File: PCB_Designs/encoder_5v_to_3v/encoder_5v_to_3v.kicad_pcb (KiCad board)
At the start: 2 copper layers, 52.1 x 57.2 mm, 17 parts, among them J1 Screw_Terminal_01x02, J2 Screw_Terminal_01x02, J3 Screw_Terminal_01x02, J4 Screw_Terminal_01x02, J5 Screw_Terminal_01x02, J6 Screw_Terminal_01x02, J7 Screw_Terminal_01x02, J8 Screw_Terminal_01x02

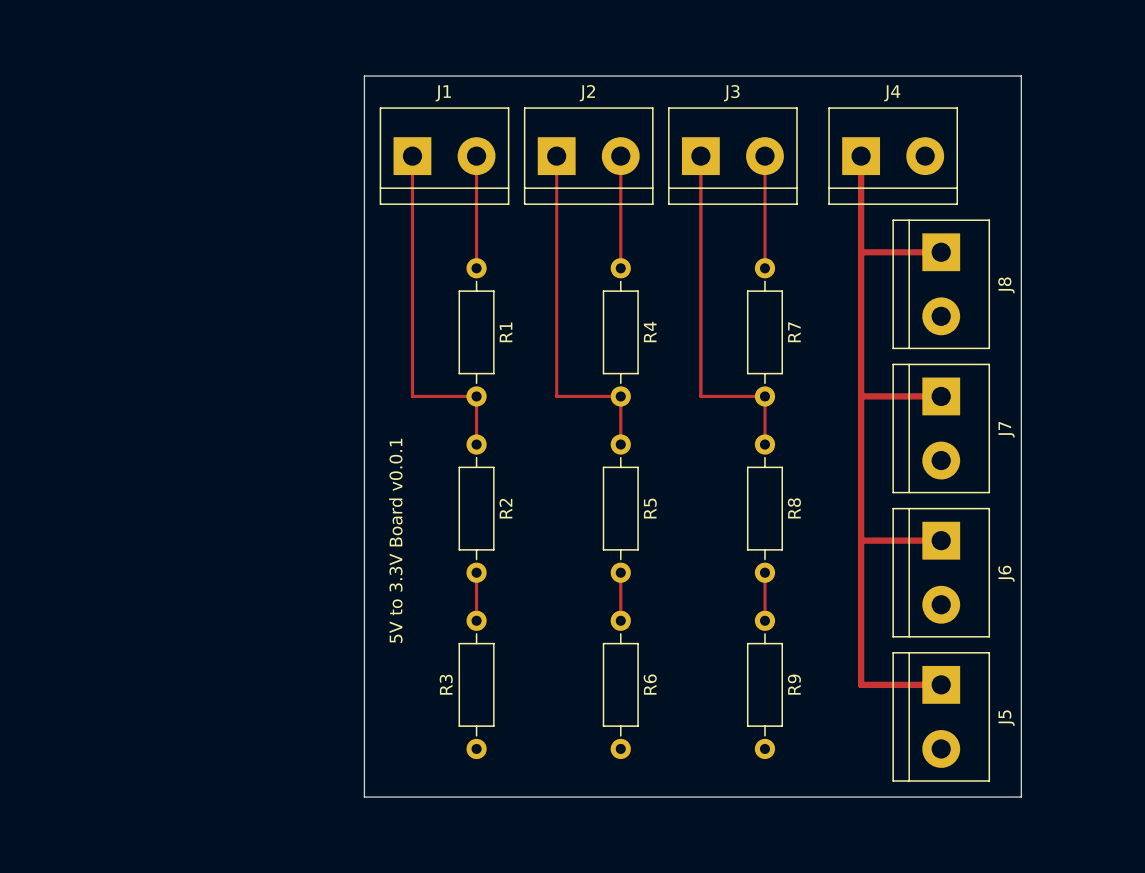
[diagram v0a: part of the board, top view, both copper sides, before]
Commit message: update PCB
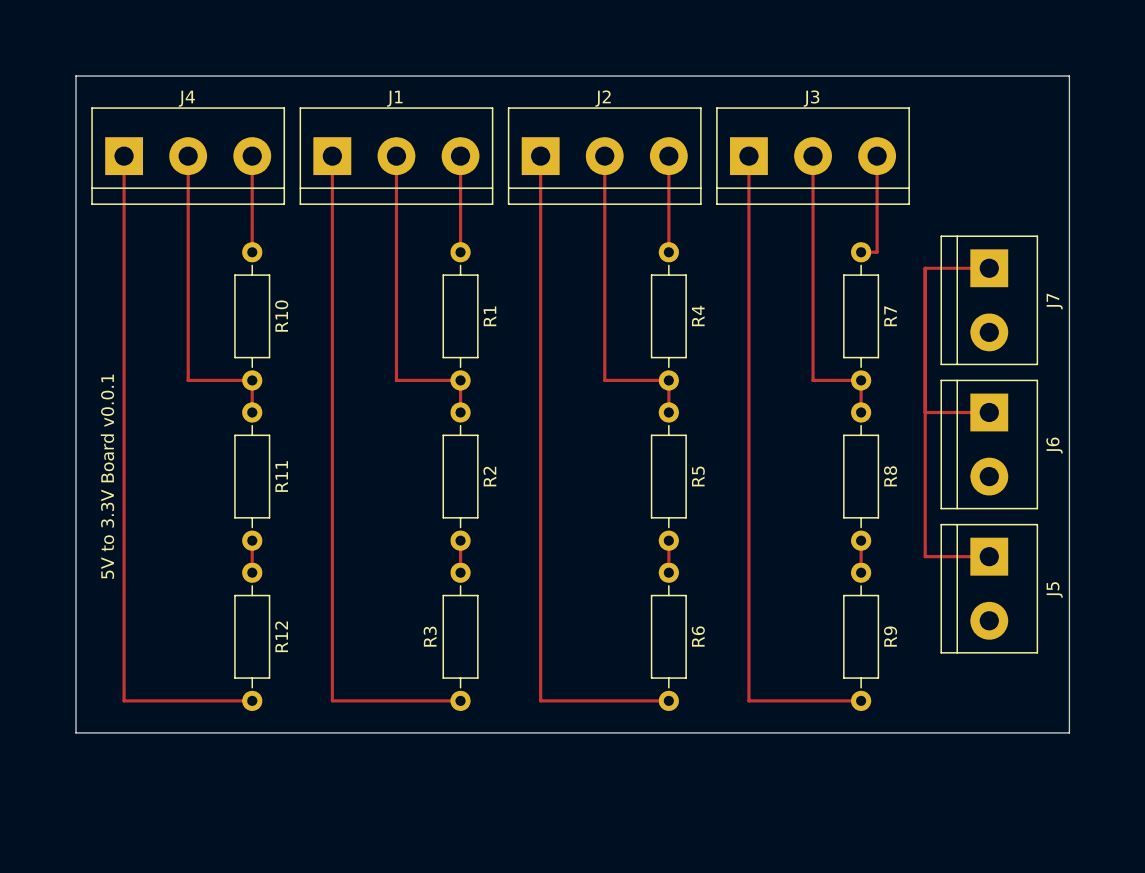
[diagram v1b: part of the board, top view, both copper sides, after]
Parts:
- removed the J5 at (134.6, 121.9)
- removed the J6 at (134.6, 110.5)
- added J4: Screw_Terminal_01x03, TerminalBlock:TerminalBlock_bornier-3_P5.08mm, F.Cu at (69.8, 80.0)
- added R10: R, Resistor_THT:R_Axial_DIN0207_L6.3mm_D2.5mm_P10.16mm_Horizontal, F.Cu at (80.0, 87.6)
- added R11: R, Resistor_THT:R_Axial_DIN0207_L6.3mm_D2.5mm_P10.16mm_Horizontal, F.Cu at (80.0, 100.3)
- added R12: R, Resistor_THT:R_Axial_DIN0207_L6.3mm_D2.5mm_P10.16mm_Horizontal, F.Cu at (80.0, 113.0)
- J1, J2, J3: value Screw_Terminal_01x02 -> Screw_Terminal_01x03; footprint TerminalBlock:TerminalBlock_bornier-2_P5.08mm -> TerminalBlock:TerminalBlock_bornier-3_P5.08mm
- moved J7 13.5 mm to (138.4, 88.9), turned to 270 degrees
- moved J5 13.3 mm to (138.4, 111.8)
- moved J6 13.3 mm to (138.4, 100.3)
- moved R9 8.52 mm to (128.3, 113.0)
- moved R8 8.03 mm to (128.3, 100.3)
- moved R7 7.73 mm to (128.3, 87.6)
- moved J1 6.35 mm to (86.4, 80.0)
- moved R6 5.39 mm to (113.0, 113.0)
- moved R5 4.58 mm to (113.0, 100.3)
- moved R3 4.02 mm to (96.5, 123.2)
- moved R4 4.02 mm to (113.0, 87.6)
- moved J3 3.81 mm to (119.4, 80.0)
- moved R2 2.84 mm to (96.5, 100.3)
- moved R1 1.80 mm to (96.5, 87.6)
- moved J2 1.27 mm to (102.9, 80.0)
- renumbered J7 to J5, J8 to J6, J4 to J7
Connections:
- J1 pad 1: Net-(J1-Pad1) -> GND
- J2 pad 1: Net-(J2-Pad1) -> GND
- J3 pad 1: Net-(J3-Pad1) -> GND
- R1 pad 1: Net-(J1-Pad2) -> Net-(J1-Pad3)
- R1 pad 2: Net-(J1-Pad1) -> Net-(J1-Pad2)
- R2 pad 1: Net-(J1-Pad1) -> Net-(J1-Pad2)
- R4 pad 1: Net-(J2-Pad2) -> Net-(J2-Pad3)
- R4 pad 2: Net-(J2-Pad1) -> Net-(J2-Pad2)
- R5 pad 1: Net-(J2-Pad1) -> Net-(J2-Pad2)
- R7 pad 1: Net-(J3-Pad2) -> Net-(J3-Pad3)
- R7 pad 2: Net-(J3-Pad1) -> Net-(J3-Pad2)
- R8 pad 1: Net-(J3-Pad1) -> Net-(J3-Pad2)
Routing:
- net GND: track 0.00 -> 212.1 mm, vias 7 -> 8
- net Net-(J3-Pad1): track 27.9 -> 0.00 mm
- net Net-(J1-Pad1): track 27.9 -> 0.00 mm
- net Net-(J2-Pad1): track 27.9 -> 0.00 mm
- net Net-(J4-Pad2): track 0.00 -> 25.4 mm
- net Net-(J5-Pad1): track 67.3 -> 49.5 mm
- net Net-(J2-Pad2): track 8.89 -> 25.4 mm
- net Net-(J1-Pad2): track 8.89 -> 25.4 mm
- net Net-(J3-Pad2): track 8.89 -> 24.1 mm
- net Net-(J3-Pad3): track 0.00 -> 8.89 mm
- net Net-(J4-Pad3): track 0.00 -> 7.62 mm
- net Net-(J2-Pad3): track 0.00 -> 7.62 mm
- net Net-(J1-Pad3): track 0.00 -> 7.62 mm
- net Net-(R11-Pad2): track 0.00 -> 2.54 mm
- net Net-(R8-Pad2): track 3.81 -> 2.54 mm
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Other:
- board size 52.1 x 57.2 mm -> 78.7 x 52.1 mm
